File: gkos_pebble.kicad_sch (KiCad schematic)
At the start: 0 parts

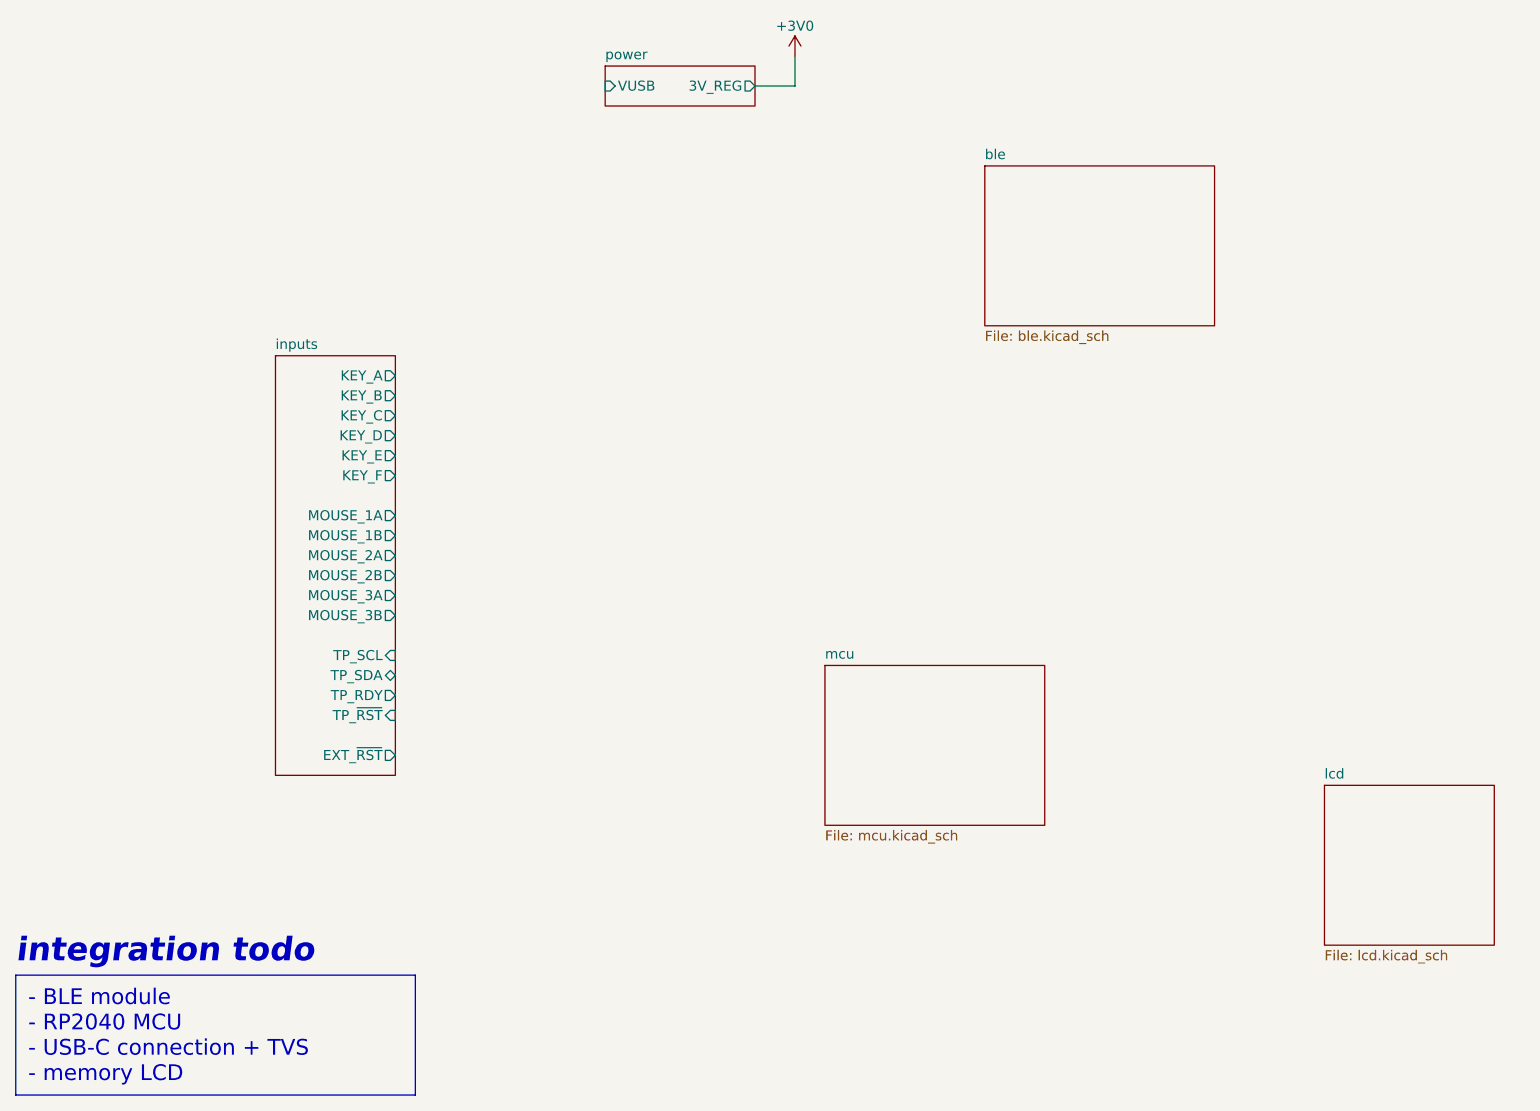
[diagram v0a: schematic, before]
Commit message: schema functionally done
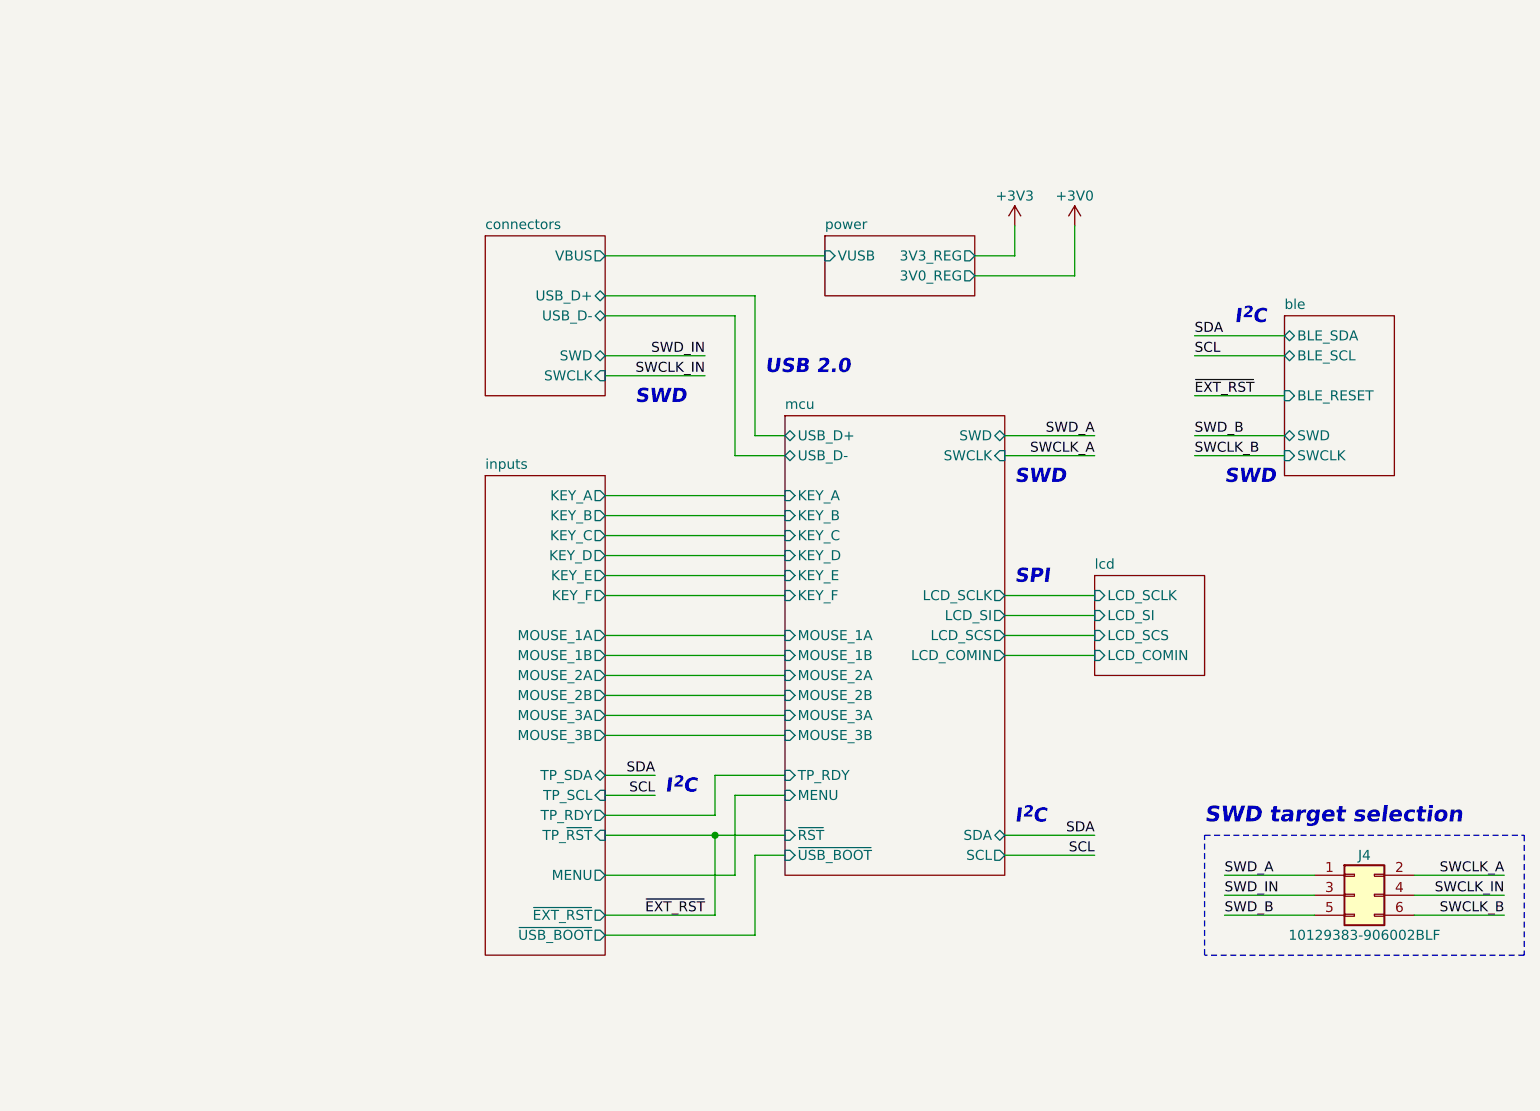
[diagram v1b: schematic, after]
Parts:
- added J4: 10129383-906002BLF, Connector_PinHeader_2.54mm:PinHeader_2x03_P2.54mm_Vertical_SMD, symbol Connector_Generic:Conn_02x03_Odd_Even
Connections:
- new net SWCLK_A: J4.2 (Pin_2)
- new net SWCLK_B: J4.6 (Pin_6)
- new net SWCLK_IN: J4.4 (Pin_4)
- new net SWD_A: J4.1 (Pin_1)
- new net SWD_B: J4.5 (Pin_5)
- new net SWD_IN: J4.3 (Pin_3)
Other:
- added sheet connectors (connectors.kicad_sch)
- sheet ble ports: added BLE_RESET, BLE_SCL, BLE_SDA, SWCLK, SWD; removed none
- sheet inputs ports: added MENU, ~{EXT_RST}, ~{USB_BOOT}; removed EXT_~{RST}
- sheet lcd ports: added LCD_COMIN, LCD_SCLK, LCD_SCS, LCD_SI; removed none
- sheet mcu ports: added KEY_A, KEY_B, KEY_C, KEY_D, KEY_E, KEY_F, LCD_COMIN, LCD_SCLK, LCD_SCS, LCD_SI, MENU, MOUSE_1A, MOUSE_1B, MOUSE_2A, MOUSE_2B, MOUSE_3A, MOUSE_3B, SCL, SDA, SWCLK, SWD, TP_RDY, USB_D+, USB_D-, ~{RST}, ~{USB_BOOT}; removed none
- sheet power ports: added 3V0_REG, 3V3_REG; removed 3V_REG
- note added: "I^{2}C"
- note added: "SPI"
- note added: "SWD"
- note added: "SWD target selection"
- note added: "USB 2.0"
- note removed: "integration todo"
